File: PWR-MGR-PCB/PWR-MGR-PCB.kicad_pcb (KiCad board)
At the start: 2 copper layers, 23 parts, among them J1 USB_C_Receptacle_USB2.0_14P, J2 Battery_1x2, J3 Conn_01x01_Pin, J4 Conn_01x01_Pin, J5 Conn_01x01_Pin, J6 Conn_01x01_Pin, U1 USBLC6-2SC6, U2 TLV75533PDBV, U3 BQ24074RGT

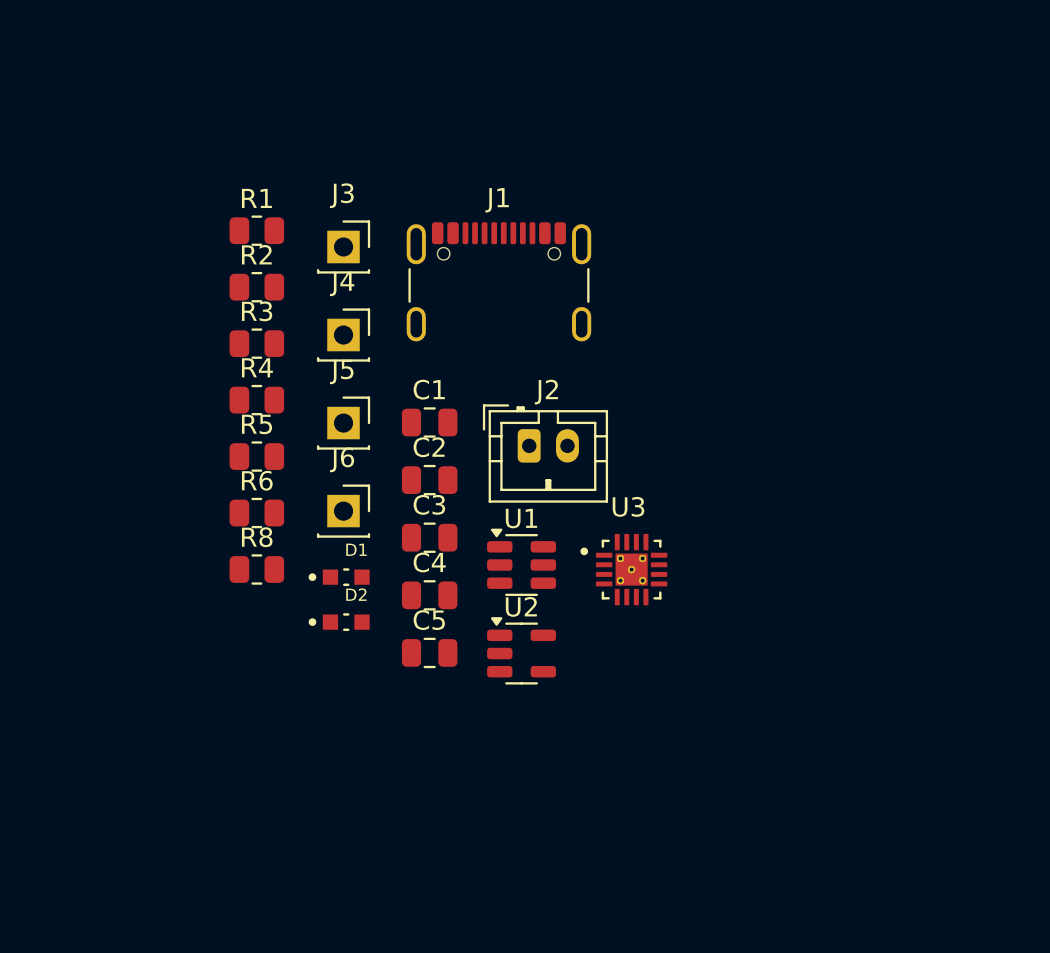
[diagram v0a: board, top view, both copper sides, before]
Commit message: Start layout
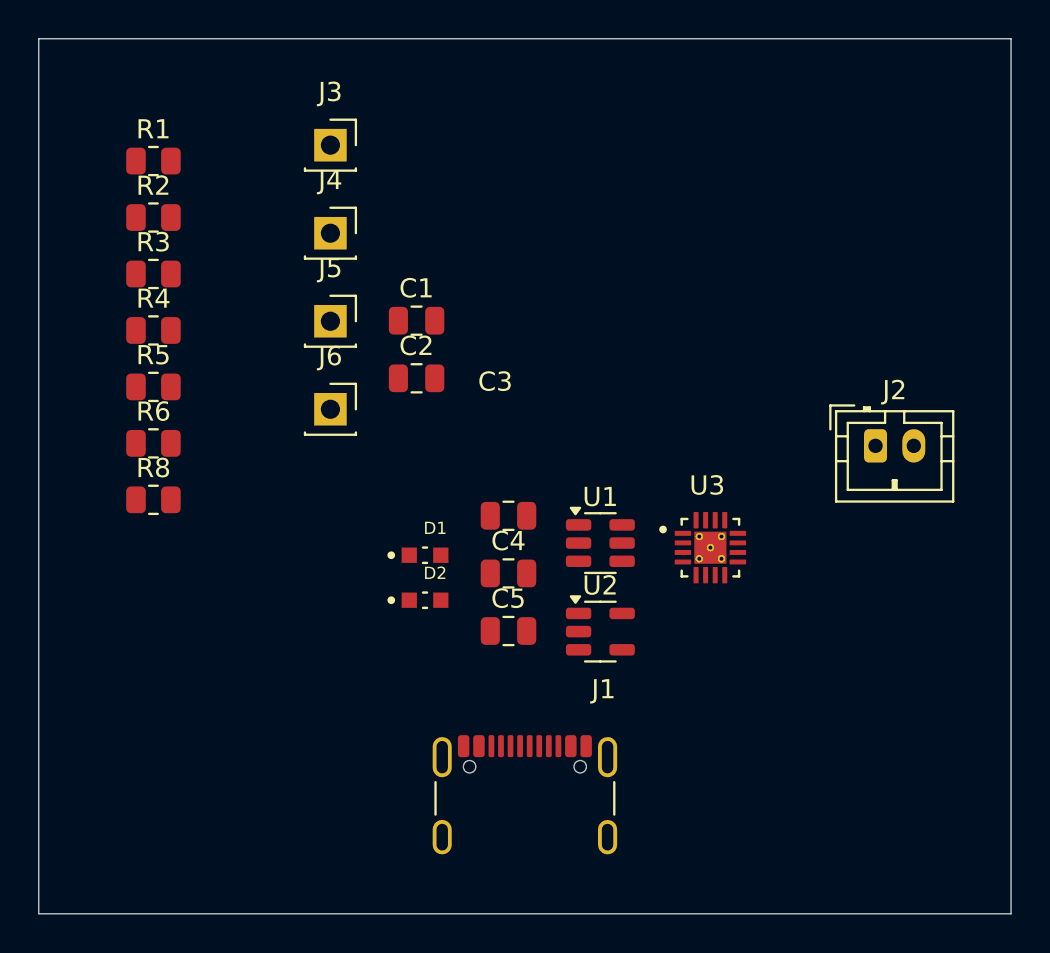
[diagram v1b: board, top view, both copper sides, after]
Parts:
- moved J1 26.8 mm to (152.4, 106.7)
- moved J2 18.1 mm to (170.7, 87.3)
- moved R2 6.51 mm to (133.0, 75.4)
- moved R3 6.51 mm to (133.0, 78.3)
- moved R4 6.51 mm to (133.0, 81.3)
- moved R5 6.51 mm to (133.0, 84.2)
- moved R8 6.51 mm to (133.0, 90.1)
- moved R1 6.51 mm to (133.0, 72.4)
- moved R6 6.51 mm to (133.0, 87.2)
- moved C1 5.36 mm to (146.7, 80.8)
- moved J3 5.36 mm to (142.2, 71.6)
- moved J5 5.36 mm to (142.2, 80.8)
- moved C2 5.36 mm to (146.7, 83.8)
- moved J4 5.36 mm to (142.2, 76.2)
- moved J6 5.36 mm to (142.2, 85.4)
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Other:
- board outline added: 50.8 x 45.7 mm
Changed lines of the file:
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@@
 	(footprint "Connector_JST:JST_PH_B2B-PH-K_1x02_P2.00mm_Vertical"
 		(layer "F.Cu")
-		(at 152.625 87.31)
+		(at 170.72 87.31)
 		(descr "JST PH series connector, B2B-PH-K (http://www.jst-mfg.com/product/pdf/eng/ePH.pdf), generated with kicad-footprint-generator")
 		(tags "connector JST PH vertical")
@@
 	(footprint "Resistor_SMD:R_0805_2012Metric"
 		(layer "F.Cu")
-		(at 138.395 84.92)
+		(at 132.9925 81.28)
 		(descr "Resistor SMD 0805 (2012 Metric), square (rectangular) end terminal, IPC-7351 nominal, (Body size source: IPC-SM-782 page 72, https://www.pcb-3d.com/wordpress/wp-content/uploads/ipc-sm-782a_amendment_1_and_2.pdf), generated with kicad-footprint-generator")
 		(tags "resistor")
@@
 	(footprint "Connector_USB:USB_C_Receptacle_GCT_USB4105-xx-A_16P_TopMnt_Horizontal"
 		(layer "F.Cu")
-		(at 151.045 79.88)
+		(at 152.4 106.68)
 		(descr "USB 2.0 Type C Receptacle, GCT, 16P, top mounted, horizontal, 5A: https://gct.co/files/drawings/usb4105.pdf")
 		(tags "USB C Type-C Receptacle SMD USB 2.0 16P 16C USB4105-15-A USB4105-15-A-060 USB4105-15-A-120 USB4105-GF-A USB4105-GF-A-060 USB4105-GF-A-120")
 		(property "Reference" "J1"
-			(at 0 -5.5 0)
+			(at 4.1175 -6.645 0)
 			(unlocked yes)
 			(layer "F.SilkS")
@@
 	(footprint "Capacitor_SMD:C_0805_2012Metric"
 		(layer "F.Cu")
-		(at 147.425 89.1)
+		(at 146.74 83.78)
 		(descr "Capacitor SMD 0805 (2012 Metric), square (rectangular) end terminal, IPC-7351 nominal, (Body size source: IPC-SM-782 page 76, https://www.pcb-3d.com/wordpress/wp-content/uploads/ipc-sm-782a_amendment_1_and_2.pdf, https://docs.google.com/spreadsheets/d/1BsfQQcO9C6DZCsRaXUlFlo91Tg2WpOkGARC1WS5S8t0/edit?usp=sharing), generated with kicad-footprint-generator")
 		(tags "capacitor")
@@
 	(footprint "BQ24074RGTR:QFN50P300X300X100-17N"
 		(layer "F.Cu")
-		(at 157.975 93.775)
+		(at 162.0925 92.63)
 		(property "Reference" "U3"
 			(at -0.165 -3.24 0)
@@
 	(footprint "Package_TO_SOT_SMD:SOT-23-5"
 		(layer "F.Cu")
-		(at 152.225 98.16)
+		(at 156.3425 97.015)
 		(descr "SOT, 5 Pin (JEDEC MO-178 Var AA https://www.jedec.org/document_search?search_api_views_fulltext=MO-178), generated with kicad-footprint-generator ipc_gullwing_generator.py")
 		(tags "SOT TO_SOT_SMD")
@@
 	(footprint "Capacitor_SMD:C_0805_2012Metric"
 		(layer "F.Cu")
-		(at 147.425 98.13)
+		(at 151.5425 96.985)
 		(descr "Capacitor SMD 0805 (2012 Metric), square (rectangular) end terminal, IPC-7351 nominal, (Body size source: IPC-SM-782 page 76, https://www.pcb-3d.com/wordpress/wp-content/uploads/ipc-sm-782a_amendment_1_and_2.pdf, https://docs.google.com/spreadsheets/d/1BsfQQcO9C6DZCsRaXUlFlo91Tg2WpOkGARC1WS5S8t0/edit?usp=sharing), generated with kicad-footprint-generator")
 		(tags "capacitor")
@@
 	(footprint "Connector_PinSocket_2.54mm:PinSocket_1x01_P2.54mm_Vertical"
 		(layer "F.Cu")
-		(at 142.925 90.72)
+		(at 142.24 85.4)
 		(descr "Through hole straight socket strip, 1x01, 2.54mm pitch, single row (from Kicad 4.0.7), script generated")
 		(tags "Through hole socket strip THT 1x01 2.54mm single row")
@@
 		)
 		(property "Value" "Conn_01x01_Pin"
-			(at 0 2.77 0)
+			(at 4.1175 1.625 0)
 			(layer "F.Fab")
 			(effects
@@
 	(footprint "Connector_PinSocket_2.54mm:PinSocket_1x01_P2.54mm_Vertical"
 		(layer "F.Cu")
-		(at 142.925 76.92)
+		(at 142.24 71.6)
 		(descr "Through hole straight socket strip, 1x01, 2.54mm pitch, single row (from Kicad 4.0.7), script generated")
 		(tags "Through hole socket strip THT 1x01 2.54mm single row")
@@
 	(footprint "Resistor_SMD:R_0805_2012Metric"
 		(layer "F.Cu")
-		(at 138.395 87.87)
+		(at 132.9925 84.23)
 		(descr "Resistor SMD 0805 (2012 Metric), square (rectangular) end terminal, IPC-7351 nominal, (Body size source: IPC-SM-782 page 72, https://www.pcb-3d.com/wordpress/wp-content/uploads/ipc-sm-782a_amendment_1_and_2.pdf), generated with kicad-footprint-generator")
 		(tags "resistor")
@@
 	(footprint "LED - SML_D12U1WT86:LED_SML-D12U1WT86"
 		(layer "F.Cu")
-		(at 143.065 96.52)
+		(at 147.1825 95.375)
 		(property "Reference" "D2"
 			(at 0.532 -1.4064 0)
@@
 	(footprint "LED - SML_D12U1WT86:LED_SML-D12U1WT86"
 		(layer "F.Cu")
-		(at 143.065 94.17)
+		(at 147.1825 93.025)
 		(property "Reference" "D1"
 			(at 0.532 -1.4064 0)
@@
 	(footprint "Connector_PinSocket_2.54mm:PinSocket_1x01_P2.54mm_Vertical"
 		(layer "F.Cu")
-		(at 142.925 81.52)
+		(at 142.24 76.2)
 		(descr "Through hole straight socket strip, 1x01, 2.54mm pitch, single row (from Kicad 4.0.7), script generated")
 		(tags "Through hole socket strip THT 1x01 2.54mm single row")
@@
 	(footprint "Resistor_SMD:R_0805_2012Metric"
 		(layer "F.Cu")
-		(at 138.395 93.77)
+		(at 132.9925 90.13)
 		(descr "Resistor SMD 0805 (2012 Metric), square (rectangular) end terminal, IPC-7351 nominal, (Body size source: IPC-SM-782 page 72, https://www.pcb-3d.com/wordpress/wp-content/uploads/ipc-sm-782a_amendment_1_and_2.pdf), generated with kicad-footprint-generator")
 		(tags "resistor")
@@
 	(footprint "Resistor_SMD:R_0805_2012Metric"
 		(layer "F.Cu")
-		(at 138.395 90.82)
+		(at 132.9925 87.18)
 		(descr "Resistor SMD 0805 (2012 Metric), square (rectangular) end terminal, IPC-7351 nominal, (Body size source: IPC-SM-782 page 72, https://www.pcb-3d.com/wordpress/wp-content/uploads/ipc-sm-782a_amendment_1_and_2.pdf), generated with kicad-footprint-generator")
 		(tags "resistor")
@@
 	(footprint "Resistor_SMD:R_0805_2012Metric"
 		(layer "F.Cu")
-		(at 138.395 76.07)
+		(at 132.9925 72.43)
 		(descr "Resistor SMD 0805 (2012 Metric), square (rectangular) end terminal, IPC-7351 nominal, (Body size source: IPC-SM-782 page 72, https://www.pcb-3d.com/wordpress/wp-content/uploads/ipc-sm-782a_amendment_1_and_2.pdf), generated with kicad-footprint-generator")
 		(tags "resistor")
@@
 	(footprint "Package_TO_SOT_SMD:SOT-23-6"
 		(layer "F.Cu")
-		(at 152.225 93.535)
+		(at 156.3425 92.39)
 		(descr "SOT, 6 Pin (JEDEC MO-178 Var AB https://www.jedec.org/document_search?search_api_views_fulltext=MO-178), generated with kicad-footprint-generator ipc_gullwing_generator.py")
 		(tags "SOT TO_SOT_SMD")
@@
 	(footprint "Capacitor_SMD:C_0805_2012Metric"
 		(layer "F.Cu")
-		(at 147.425 92.11)
+		(at 151.5425 90.965)
 		(descr "Capacitor SMD 0805 (2012 Metric), square (rectangular) end terminal, IPC-7351 nominal, (Body size source: IPC-SM-782 page 76, https://www.pcb-3d.com/wordpress/wp-content/uploads/ipc-sm-782a_amendment_1_and_2.pdf, https://docs.google.com/spreadsheets/d/1BsfQQcO9C6DZCsRaXUlFlo91Tg2WpOkGARC1WS5S8t0/edit?usp=sharing), generated with kicad-footprint-generator")
 		(tags "capacitor")
 		(property "Reference" "C3"
-			(at 0 -1.68 0)
+			(at -0.685 -7 0)
 			(layer "F.SilkS")
 			(effects
@@
 	(footprint "Resistor_SMD:R_0805_2012Metric"
 		(layer "F.Cu")
-		(at 138.395 81.97)
+		(at 132.9925 78.33)
 		(descr "Resistor SMD 0805 (2012 Metric), square (rectangular) end terminal, IPC-7351 nominal, (Body size source: IPC-SM-782 page 72, https://www.pcb-3d.com/wordpress/wp-content/uploads/ipc-sm-782a_amendment_1_and_2.pdf), generated with kicad-footprint-generator")
 		(tags "resistor")
@@
 	(footprint "Connector_PinSocket_2.54mm:PinSocket_1x01_P2.54mm_Vertical"
 		(layer "F.Cu")
-		(at 142.925 86.12)
+		(at 142.24 80.8)
 		(descr "Through hole straight socket strip, 1x01, 2.54mm pitch, single row (from Kicad 4.0.7), script generated")
 		(tags "Through hole socket strip THT 1x01 2.54mm single row")
@@
 	(footprint "Capacitor_SMD:C_0805_2012Metric"
 		(layer "F.Cu")
-		(at 147.425 86.09)
+		(at 146.74 80.77)
 		(descr "Capacitor SMD 0805 (2012 Metric), square (rectangular) end terminal, IPC-7351 nominal, (Body size source: IPC-SM-782 page 76, https://www.pcb-3d.com/wordpress/wp-content/uploads/ipc-sm-782a_amendment_1_and_2.pdf, https://docs.google.com/spreadsheets/d/1BsfQQcO9C6DZCsRaXUlFlo91Tg2WpOkGARC1WS5S8t0/edit?usp=sharing), generated with kicad-footprint-generator")
 		(tags "capacitor")
@@
 	(footprint "Resistor_SMD:R_0805_2012Metric"
 		(layer "F.Cu")
-		(at 138.395 79.02)
+		(at 132.9925 75.38)
 		(descr "Resistor SMD 0805 (2012 Metric), square (rectangular) end terminal, IPC-7351 nominal, (Body size source: IPC-SM-782 page 72, https://www.pcb-3d.com/wordpress/wp-content/uploads/ipc-sm-782a_amendment_1_and_2.pdf), generated with kicad-footprint-generator")
 		(tags "resistor")
@@
 	(footprint "Capacitor_SMD:C_0805_2012Metric"
 		(layer "F.Cu")
-		(at 147.425 95.12)
+		(at 151.5425 93.975)
 		(descr "Capacitor SMD 0805 (2012 Metric), square (rectangular) end terminal, IPC-7351 nominal, (Body size source: IPC-SM-782 page 76, https://www.pcb-3d.com/wordpress/wp-content/uploads/ipc-sm-782a_amendment_1_and_2.pdf, https://docs.google.com/spreadsheets/d/1BsfQQcO9C6DZCsRaXUlFlo91Tg2WpOkGARC1WS5S8t0/edit?usp=sharing), generated with kicad-footprint-generator")
 		(tags "capacitor")
@@
 		)
 	)
+	(gr_line
+		(start 127 66.04)
+		(end 127 111.76)
+		(stroke
+			(width 0.05)
+			(type default)
+		)
+		(layer "Edge.Cuts")
+	)
+	(gr_line
+		(start 177.8 66.04)
+		(end 127 66.04)
+		(stroke
+			(width 0.05)
+			(type default)
+		)
+		(layer "Edge.Cuts")
+	)
+	(gr_line
+		(start 127 111.76)
+		(end 177.8 111.76)
+		(stroke
+			(width 0.05)
+			(type default)
+		)
+		(layer "Edge.Cuts")
+	)
+	(gr_line
+		(start 177.8 111.76)
+		(end 177.8 66.04)
+		(stroke
+			(width 0.05)
+			(type default)
+		)
+		(layer "Edge.Cuts")
+	)
 	(embedded_fonts no)
